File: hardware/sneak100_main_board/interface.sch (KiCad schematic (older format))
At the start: 13 parts, among them J1 Conn_01x03, SW1 SW_Push, SW2 SW_Push

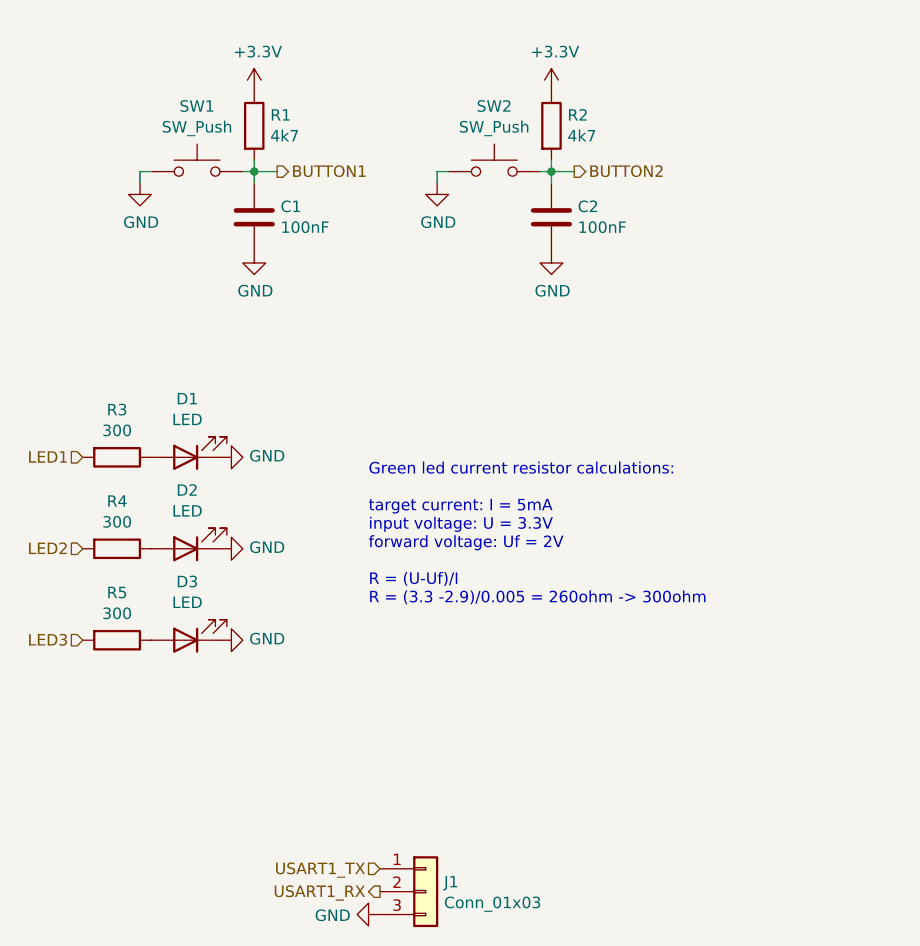
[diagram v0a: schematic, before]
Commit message: motors circuit scheme
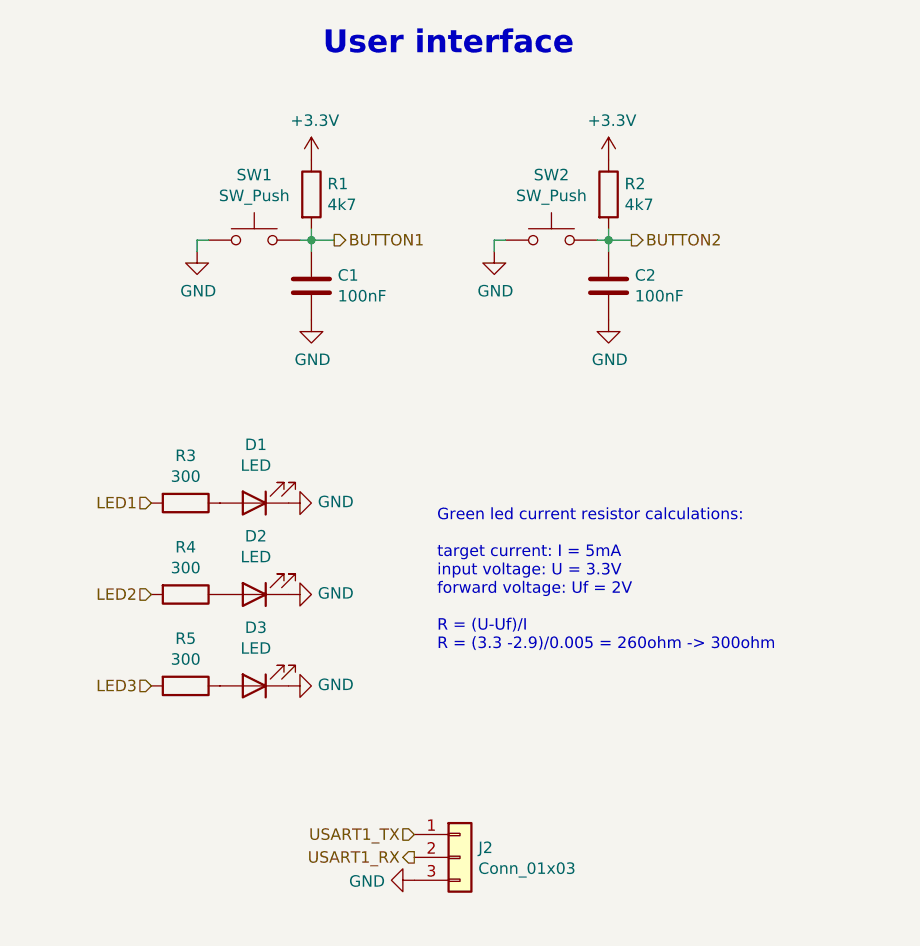
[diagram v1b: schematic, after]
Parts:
- C1, C2: footprint (none) -> Capacitor_SMD:C_0805_2012Metric
- D1, D2, D3: footprint (none) -> LED_SMD:LED_0805_2012Metric
- J2: renamed from J1; footprint (none) -> Connector_PinHeader_2.54mm:PinHeader_1x03_P2.54mm_Vertical
- R1, R2, R3, R4, R5: footprint (none) -> Resistor_SMD:R_0805_2012Metric
- SW1, SW2: footprint (none) -> Button_Switch_SMD:SW_SPST_FSMSM
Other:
- note added: "User interface"
- moved on the sheet: C1, C2, D1, D2, D3, J2, R1, R2, R3, R4, R5, SW1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
